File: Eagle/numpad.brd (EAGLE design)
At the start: 95 x 99 mm, 36 parts, among them SW1 SWITCH-SMD-SCHURTER-1241.1612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, U1 PROMICRO

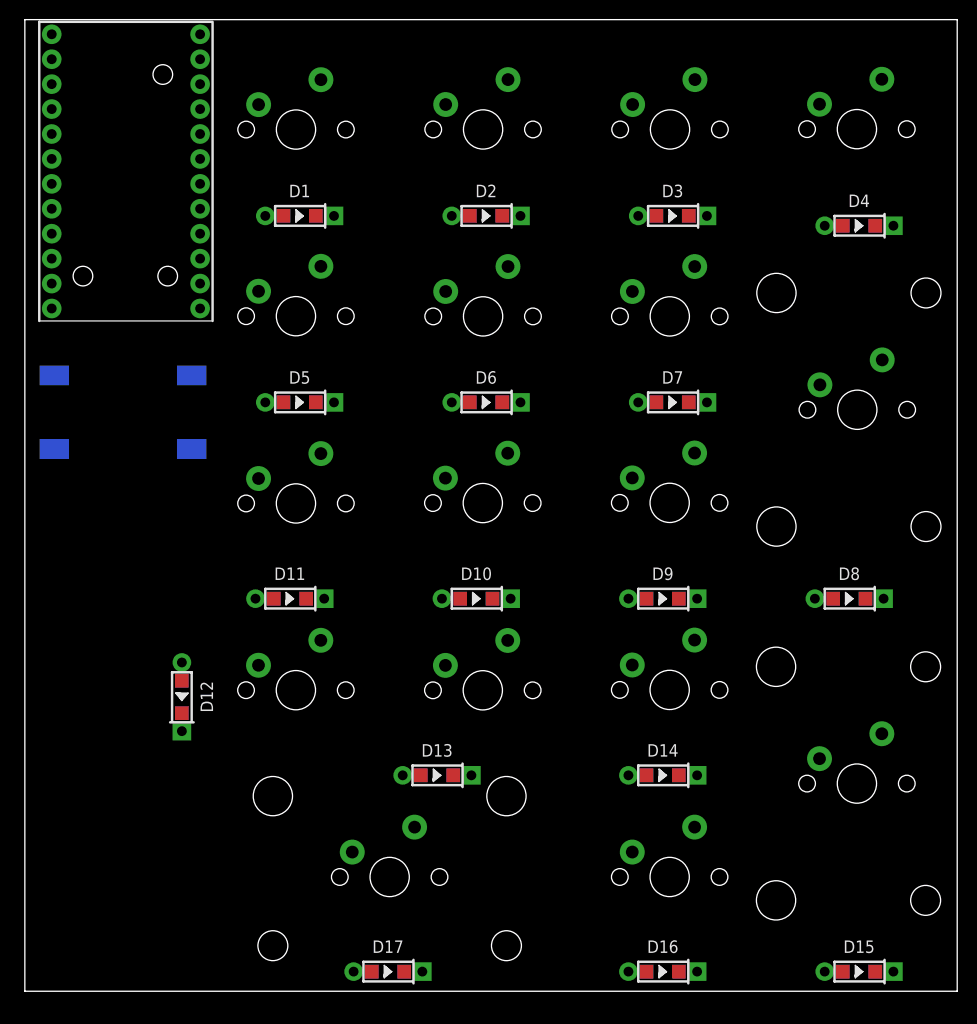
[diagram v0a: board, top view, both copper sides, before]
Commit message: added hole
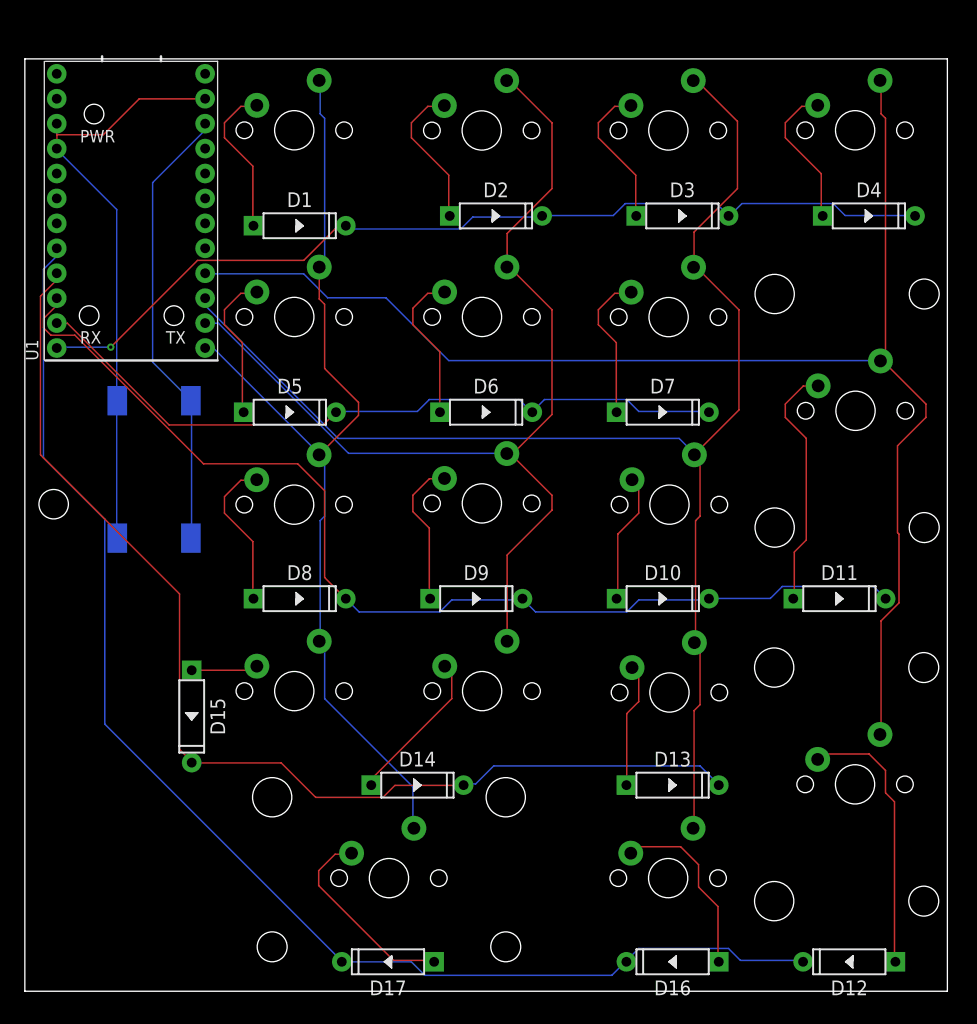
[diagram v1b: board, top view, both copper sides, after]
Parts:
- D1, D10, D11, D12, D13, D14, D15, D16, D17, D2, D3, D4, D5, D6, D7, D8, D9: value (none) -> 1N4148; device Components:DIODE_HAND -> Components:DO-35
- moved D12 73.2 mm to (85.0, 9.00), turned to 180 degrees
- moved D15 72.8 mm to (18.0, 34.0), turned to 270 degrees
- moved D11 56.0 mm to (84.0, 46.0)
- moved D8 56.0 mm to (29.0, 46.0)
- moved D14 25.0 mm to (41.0, 27.0)
- moved D13 24.0 mm to (67.0, 27.0)
- moved D10 19.0 mm to (66.0, 46.0)
- moved D9 19.0 mm to (47.0, 46.0)
- moved SW1 6.64 mm to (14.2, 59.2), turned to 270 degrees
- moved U1 4.08 mm to (11.9, 85.5), flipped to the top
- moved D16 1.41 mm to (67.0, 9.00), turned to 180 degrees
- moved D4 1.41 mm to (87.0, 85.0)
- moved D5 1.41 mm to (28.0, 65.0)
- moved D7 1.41 mm to (66.0, 65.0)
- moved D1 1.00 mm to (29.0, 84.0)
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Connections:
- net N$27 renamed COL2
- net N$30 renamed COL3
- net N$7 renamed COL0
- net N$9 renamed COL1
- removed net N$16: D12.A1, D12.A2, D12.A3, U$29.MX1
- removed net N$22: D15.C1, D15.C2, D15.C3, D16.C1, D16.C2, D16.C3, D17.C1, D17.C2, D17.C3, U1.5
- removed net N$23: D12.C1, D12.C2, D12.C3, D13.C1, D13.C2, D13.C3, D14.C1, D14.C2, D14.C3, U1.6
- removed net N$24: D10.C1, D10.C2, D10.C3, D11.C1, D11.C2, D11.C3, D9.C1, D9.C2, D9.C3, U1.7
- removed net N$26: D5.C1, D5.C2, D5.C3, D6.C1, D6.C2, D6.C3, D7.C1, D7.C2, D7.C3, D8.C1, D8.C2, D8.C3, U1.8
- new net ROW0: D1.C, D2.C, D3.C, D4.C, U1.9
- new net ROW1: D5.C, D6.C, D7.C, U1.8
- new net ROW2: D10.C, D11.C, D8.C, D9.C, U1.7
- new net ROW3: D13.C, D14.C, D15.C, U1.6
- new net ROW4: D12.C, D16.C, D17.C, U1.5
- net N$10: now also D6.A; no longer D6.A1, D6.A2, D6.A3
- net N$11: now also D7.A; no longer D7.A1, D7.A2, D7.A3
- net N$12: now also D11.A; no longer D8.A1, D8.A2, D8.A3
- net N$13: now also D10.A; no longer D9.A1, D9.A2, D9.A3
- net N$14: now also D9.A; no longer D10.A1, D10.A2, D10.A3
- net N$15: now also D8.A; no longer D11.A1, D11.A2, D11.A3
- net N$17: now also D14.A; no longer D13.A1, D13.A2, D13.A3
- net N$18: now also D13.A; no longer D14.A1, D14.A2, D14.A3
- net N$19: now also D16.A; no longer D16.A1, D16.A2, D16.A3
- net N$2: now also D1.A; no longer D1.A1, D1.A2, D1.A3
- net N$20: now also D17.A; no longer D17.A1, D17.A2, D17.A3
- net N$21: now also D12.A; no longer D15.A1, D15.A2, D15.A3
- net N$3: now also D2.A; no longer D2.A1, D2.A2, D2.A3
- net N$4: now also D3.A; no longer D3.A1, D3.A2, D3.A3
- net N$5: now also D4.A; no longer D4.A1, D4.A2, D4.A3
- net N$6: now also D15.A, U$29.MX1; no longer D1.C1, D1.C2, D1.C3, D2.C1, D2.C2, D2.C3, D3.C1, D3.C2, D3.C3, D4.C1, D4.C2, D4.C3, U1.9
- net N$8: now also D5.A; no longer D5.A1, D5.A2, D5.A3
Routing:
- net COL3: track 0.00 -> 144.4 mm
- net COL2: track 0.00 -> 142.1 mm
- net ROW4: track 0.00 -> 135.2 mm
- net ROW3: track 0.00 -> 114.3 mm
- net ROW2: track 0.00 -> 109.3 mm
- net COL1: track 0.00 -> 105.8 mm
- net COL0: track 0.00 -> 101.0 mm
- net ROW0: track 0.00 -> 95.4 mm, vias 0 -> 1
- net ROW1: track 0.00 -> 73.4 mm
- net GND: track 0.00 -> 61.4 mm
- net N$1: track 0.00 -> 46.1 mm
- net N$21: track 0.00 -> 27.8 mm
- net N$12: track 0.00 -> 25.4 mm
- net N$20: track 0.00 -> 20.7 mm
- net N$19: track 0.00 -> 18.7 mm
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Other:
- board size 95 x 99 mm -> 94 x 95 mm
